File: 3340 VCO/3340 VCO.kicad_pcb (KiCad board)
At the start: 2 copper layers, 60.6 x 104.5 mm, 74 parts, among them J1 Conn_02x05_Odd_Even, J2 Conn_01x19, U1 TL072, U2 TL072, U3 TL072, U4 AS3340, U6 LM7905_TO220

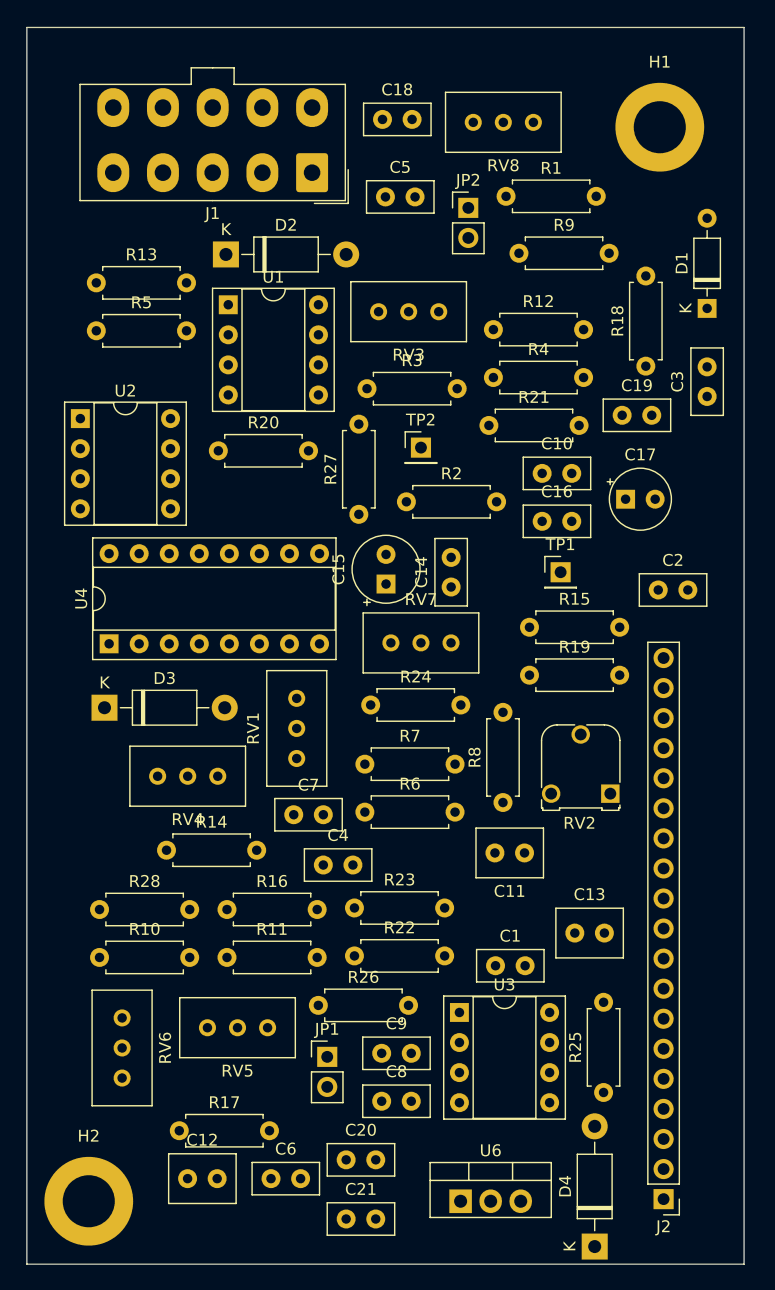
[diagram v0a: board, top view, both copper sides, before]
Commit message: Finish VCO
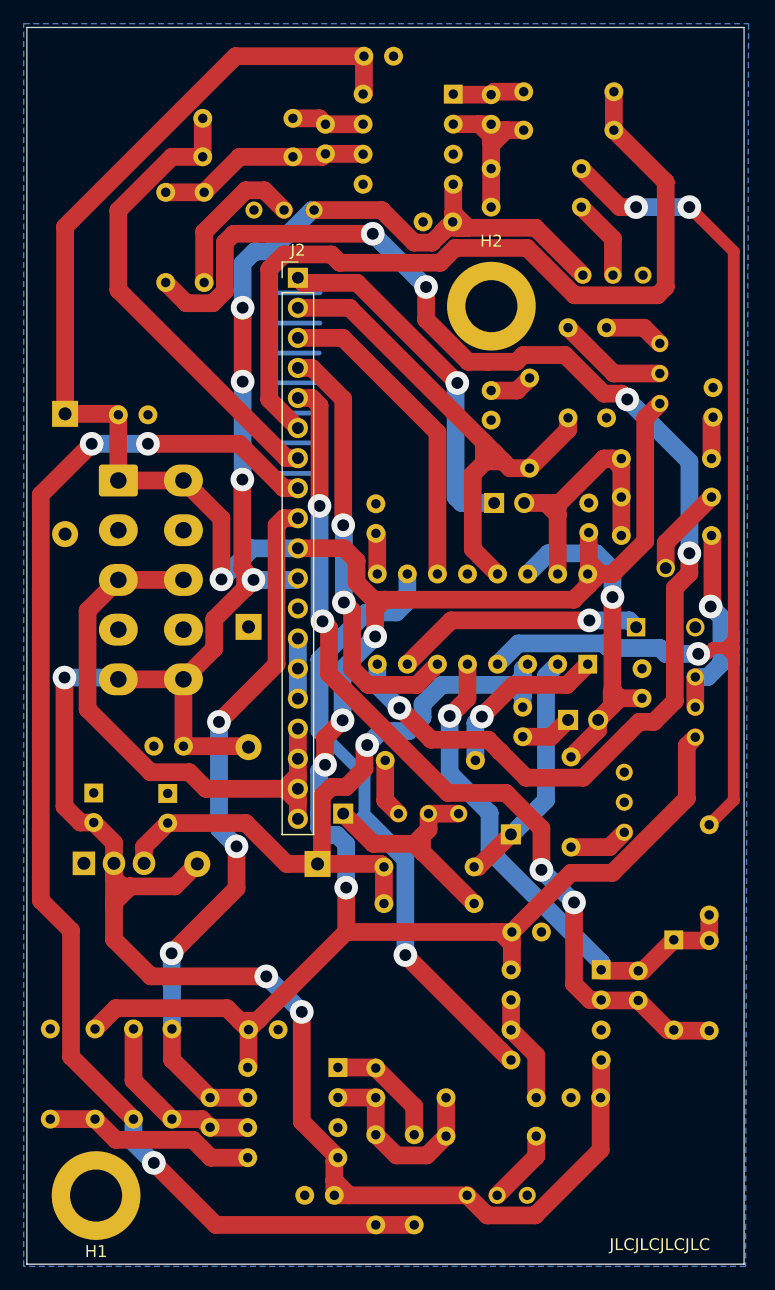
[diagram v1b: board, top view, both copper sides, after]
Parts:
- C1, C10, C11, C12, C13, C14, C15, C16, C17, C18, C19, C2, C20, C21, C3, C4, C5, C6, C7, C8, C9, D1, D2, D3, D4, JP1, JP2, R1, R10, R11, R12, R13, R14, R15, R16, R17, R18, R19, R2, R20, R21, R22, R23, R24, R25, R26, R27, R28, R3, R4, R5, R6, R7, R8, R9, RV1, RV2, RV3, RV4, RV5, RV6, RV7, RV8, TP1, TP2, U1, U2, U3, U4, U6: moved to B.Cu
- J1: value Conn_02x05_Odd_Even -> Conn_02x05_Top_Bottom; moved to B.Cu
- moved H1 102.1 mm to (120.1, 134.8)
- moved C6 95.4 mm to (145.2, 38.5), turned to 180 degrees
- moved RV8 90.8 mm to (156.6, 134.8), turned to 0 degrees
- moved J2 83.8 mm to (137.2, 57.2), turned to 0 degrees
- moved H2 82.9 mm to (153.5, 59.6)
- moved RV6 80.9 mm to (166.3, 57.0), turned to 0 degrees
- moved R22 74.4 mm to (156.2, 41.5)
- moved R23 66.9 mm to (136.8, 43.8), turned to 180 degrees
- moved R18 65.7 mm to (157.3, 129.8), turned to 180 degrees
- moved R14 64.7 mm to (161.1, 51.2), turned to 180 degrees
- moved U1 64.4 mm to (162.8, 115.7), turned to 180 degrees
- moved R21 60.7 mm to (143.8, 129.6), turned to -90 degrees
- moved R4 58.1 mm to (171.9, 120.8), turned to 90 degrees
- moved D1 53.4 mm to (168.9, 113.2), turned to -90 degrees
- moved R9 53.1 mm to (144.4, 107.0)
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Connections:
- J1 pad 2: +12V -> GND
- J1 pad 3: GND -> Chassis
- J1 pad 5: Chassis -> -12V
- J1 pad 6: Chassis -> +12V
- J1 pad 8: GND -> Chassis
- J1 pad 9: -12V -> GND
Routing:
- net +12V: track 0.00 -> 244.8 mm, vias 0 -> 5
- net -12V: track 0.00 -> 212.7 mm, vias 0 -> 7
- net Net-(U4-VSO): track 0.00 -> 113.5 mm, vias 0 -> 5
- net /TRI: track 0.00 -> 109.6 mm, vias 0 -> 3
- net Net-(U4-VP): track 0.00 -> 89.5 mm, vias 0 -> 3
- net /PWM: track 0.00 -> 75.8 mm, vias 0 -> 4
- net /PULSE: track 0.00 -> 69.5 mm
- net -5V: track 0.00 -> 63.4 mm, vias 0 -> 1
- net /LED: track 0.00 -> 59.8 mm, vias 0 -> 3
- net Net-(U1B-+): track 0.00 -> 52.4 mm, vias 0 -> 1
- net Chassis: track 0.00 -> 48.9 mm
- net /FM_LIN: track 0.00 -> 45.9 mm
- net Net-(D1-K): track 0.00 -> 44.2 mm, vias 0 -> 1
- net /RAMP: track 0.00 -> 40.0 mm
- net /HS: track 0.00 -> 36.5 mm, vias 0 -> 2
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- added copper zone on B.Cu, net GND
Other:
- board text added: "JLCJLCJLCJLC"
- board text added: "VCO V1 Matthew Taylor"
